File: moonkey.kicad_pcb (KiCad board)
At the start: 2 copper layers, 34 parts

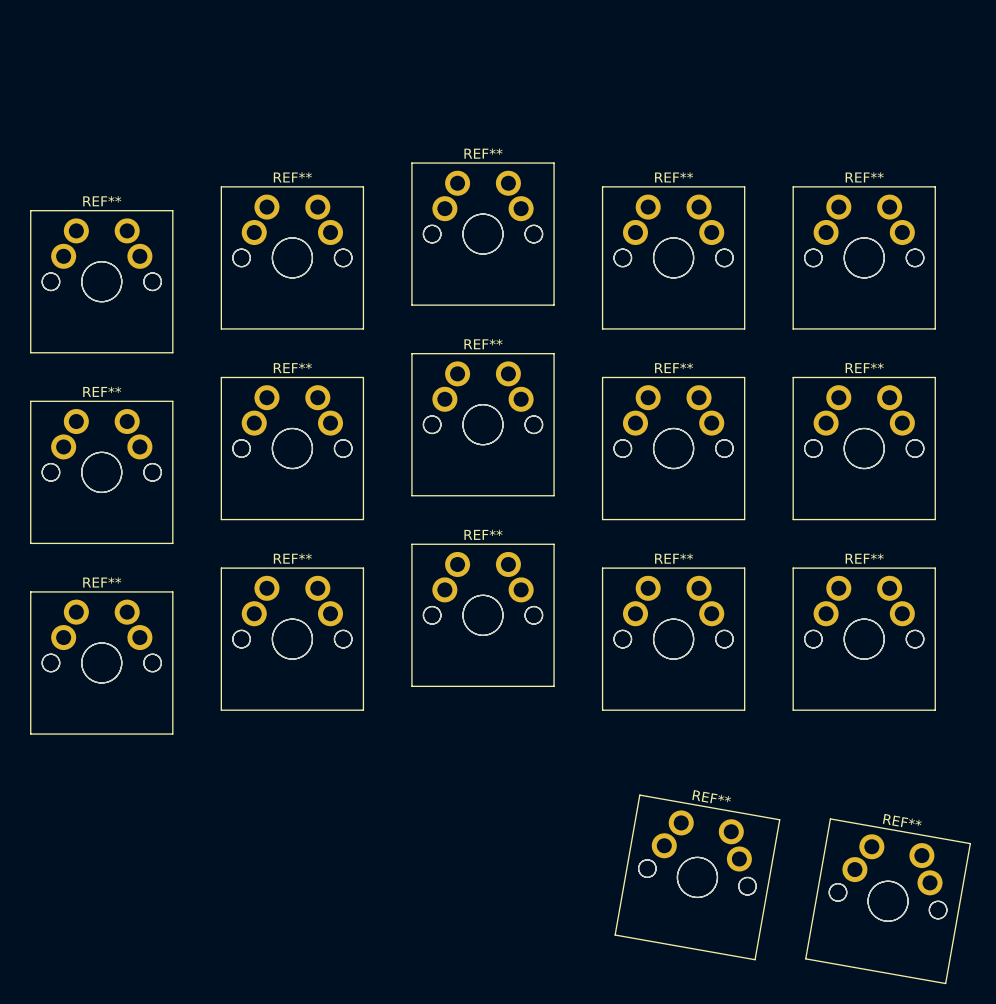
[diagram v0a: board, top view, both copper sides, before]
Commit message: update
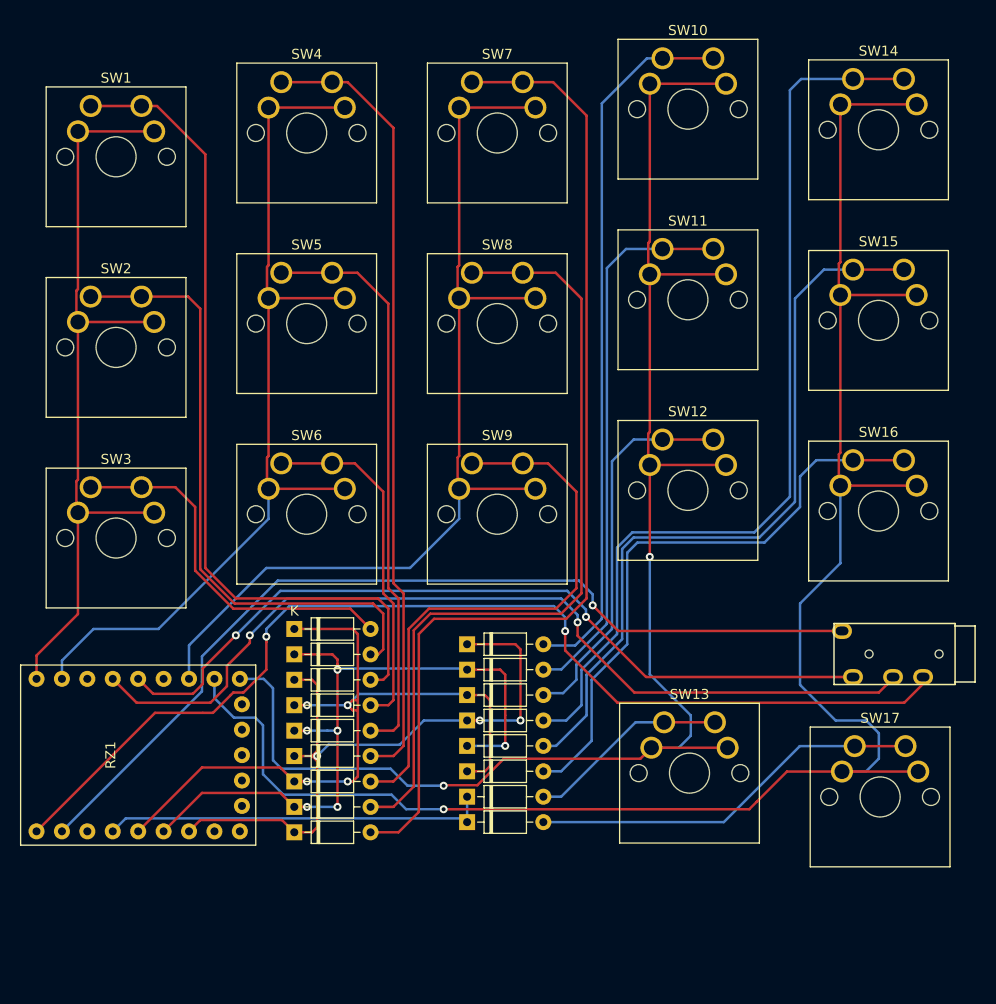
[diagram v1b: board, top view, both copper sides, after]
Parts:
- removed REF** (x32): SW_Cherry_MX_PCB_1.00u, Switch_Keyboard_Cherry_MX:SW_Cherry_MX_PCB_1.00u
- removed REF** (x2): SW_Cherry_MX_PCB_1.50u_90deg, Switch_Keyboard_Cherry_MX:SW_Cherry_MX_PCB_1.50u_90deg
- added D1: 1N4148, Diode_THT:D_DO-35_SOD27_P7.62mm_Horizontal, F.Cu at (128.8, 118.4)
- added D10: 1N4148, Diode_THT:D_DO-35_SOD27_P7.62mm_Horizontal, F.Cu at (146.1, 114.8)
- added D11: 1N4148, Diode_THT:D_DO-35_SOD27_P7.62mm_Horizontal, F.Cu at (146.1, 117.3)
- added D12: 1N4148, Diode_THT:D_DO-35_SOD27_P7.62mm_Horizontal, F.Cu at (146.1, 119.9)
- added D13: 1N4148, Diode_THT:D_DO-35_SOD27_P7.62mm_Horizontal, F.Cu at (146.1, 130.0)
- added D14: 1N4148, Diode_THT:D_DO-35_SOD27_P7.62mm_Horizontal, F.Cu at (146.1, 122.4)
- added D15: 1N4148, Diode_THT:D_DO-35_SOD27_P7.62mm_Horizontal, F.Cu at (146.1, 125.0)
- added D16: 1N4148, Diode_THT:D_DO-35_SOD27_P7.62mm_Horizontal, F.Cu at (146.1, 127.5)
- added D17: 1N4148, Diode_THT:D_DO-35_SOD27_P7.62mm_Horizontal, F.Cu at (146.1, 132.6)
- added D2: 1N4148, Diode_THT:D_DO-35_SOD27_P7.62mm_Horizontal, F.Cu at (128.8, 115.8)
- added D3: 1N4148, Diode_THT:D_DO-35_SOD27_P7.62mm_Horizontal, F.Cu at (128.8, 113.3)
- added D4: 1N4148, Diode_THT:D_DO-35_SOD27_P7.62mm_Horizontal, F.Cu at (128.8, 126.0)
- added D5: 1N4148, Diode_THT:D_DO-35_SOD27_P7.62mm_Horizontal, F.Cu at (128.8, 123.4)
- added D6: 1N4148, Diode_THT:D_DO-35_SOD27_P7.62mm_Horizontal, F.Cu at (128.8, 120.9)
- added D7: 1N4148, Diode_THT:D_DO-35_SOD27_P7.62mm_Horizontal, F.Cu at (128.8, 133.6)
- added D8: 1N4148, Diode_THT:D_DO-35_SOD27_P7.62mm_Horizontal, F.Cu at (128.8, 131.1)
- added D9: 1N4148, Diode_THT:D_DO-35_SOD27_P7.62mm_Horizontal, F.Cu at (128.8, 128.5)
- added J1: AudioJack4, moonkey:PJ320A, F.Cu at (194.8, 115.8)
- added RZ1: RP2040-Zero, moonkey:RP2040, F.Cu at (124.9, 134.9)
- added SW1: SW_Push, moonkey:Cherry_1u_rev, F.Cu at (113.5, 61.0)
- added SW10: SW_Push, moonkey:Cherry_1u_rev, F.Cu at (170.7, 56.3)
- added SW11: SW_Push, moonkey:Cherry_1u_rev, F.Cu at (170.7, 75.3)
- added SW12: SW_Push, moonkey:Cherry_1u_rev, F.Cu at (170.7, 94.4)
- added SW13: SW_Push, moonkey:Cherry_1u_rev, F.Cu at (170.8, 122.6)
- added SW14: SW_Push, moonkey:Cherry_1u_rev, F.Cu at (189.7, 58.3)
- added SW15: SW_Push, moonkey:Cherry_1u_rev, F.Cu at (189.7, 77.4)
- added SW16: SW_Push, moonkey:Cherry_1u_rev, F.Cu at (189.7, 96.4)
- added SW17: SW_Push, moonkey:Cherry_1u_rev, F.Cu at (189.9, 125.0)
- added SW2: SW_Push, moonkey:Cherry_1u_rev, F.Cu at (113.5, 80.1)
- added SW3: SW_Push, moonkey:Cherry_1u_rev, F.Cu at (113.5, 99.1)
- added SW4: SW_Push, moonkey:Cherry_1u_rev, F.Cu at (132.6, 58.6)
- added SW5: SW_Push, moonkey:Cherry_1u_rev, F.Cu at (132.6, 77.7)
- added SW6: SW_Push, moonkey:Cherry_1u_rev, F.Cu at (132.6, 96.7)
- added SW7: SW_Push, moonkey:Cherry_1u_rev, F.Cu at (151.6, 58.6)
- added SW8: SW_Push, moonkey:Cherry_1u_rev, F.Cu at (151.6, 77.7)
- added SW9: SW_Push, moonkey:Cherry_1u_rev, F.Cu at (151.6, 96.7)
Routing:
- net ROW4: track 0.00 -> 180.7 mm, vias 0 -> 1
- net ROW3: track 0.00 -> 153.7 mm, vias 0 -> 2
- net +5V: track 0.00 -> 108.0 mm, vias 0 -> 2
- net Net-(D7-Pad2): track 0.00 -> 102.8 mm
- net ROW2: track 0.00 -> 99.8 mm
- net Net-(D14-Pad2): track 0.00 -> 93.5 mm
- net Earth: track 0.00 -> 93.1 mm, vias 0 -> 1
- net ROW1: track 0.00 -> 92.6 mm
- net SPI0_TX: track 0.00 -> 90.8 mm, vias 0 -> 2
- net Net-(D1-Pad2): track 0.00 -> 83.4 mm
- net SPI0_RX: track 0.00 -> 81.5 mm, vias 0 -> 2
- net Net-(D8-Pad2): track 0.00 -> 80.6 mm
- net ROW0: track 0.00 -> 79.5 mm
- net Net-(D4-Pad2): track 0.00 -> 79.0 mm
- net COL2: track 0.00 -> 78.0 mm, vias 0 -> 4
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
